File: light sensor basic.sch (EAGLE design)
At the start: 1 part

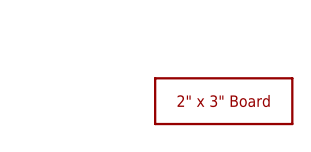
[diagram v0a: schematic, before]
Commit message: test
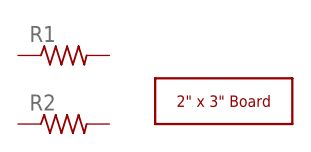
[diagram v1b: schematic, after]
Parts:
- added R1, R2: (no value), rcl:R-US_R1206
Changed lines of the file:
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@@
 <parts>
 <part name="U$1" library="voltera_community_lib" deviceset="2X3_BOARD" device="_V2"/>
+<part name="R1" library="rcl" library_urn="urn:adsk.eagle:library:334" deviceset="R-US_" device="R1206" package3d_urn="urn:adsk.eagle:package:23540/2"/>
+<part name="R2" library="rcl" library_urn="urn:adsk.eagle:library:334" deviceset="R-US_" device="R1206" package3d_urn="urn:adsk.eagle:package:23540/2"/>
 </parts>
 <sheets>
@@
 <instances>
 <instance part="U$1" gate="G$1" x="25.4" y="25.4" smashed="yes"/>
+<instance part="R1" gate="G$1" x="7.62" y="30.48" smashed="yes">
+<attribute name="NAME" x="3.81" y="31.9786" size="1.778" layer="95"/>
+<attribute name="VALUE" x="3.81" y="27.178" size="1.778" layer="96"/>
+</instance>
+<instance part="R2" gate="G$1" x="7.62" y="22.86" smashed="yes">
+<attribute name="NAME" x="3.81" y="24.3586" size="1.778" layer="95"/>
+<attribute name="VALUE" x="3.81" y="19.558" size="1.778" layer="96"/>
+</instance>
 </instances>
 <busses>
@@
 </schematic>
 </drawing>
+<compatibility>
+<note version="8.2" severity="warning">
+Since Version 8.2, EAGLE supports online libraries. The ids
+of those online libraries will not be understood (or retained)
+with this version.
+</note>
+<note version="8.3" severity="warning">
+Since Version 8.3, EAGLE supports URNs for individual library
+assets (packages, symbols, and devices). The URNs of those assets
+will not be understood (or retained) with this version.
+</note>
+<note version="8.3" severity="warning">
+Since Version 8.3, EAGLE supports the association of 3D packages
+with devices in libraries, schematics, and board files. Those 3D
+packages will not be understood (or retained) with this version.
+</note>
+<note version="8.4" severity="warning">
+Since Version 8.4, EAGLE supports properties for SPICE simulation.
+Probes in schematics and SPICE mapping objects found in parts and library devices
+will not be understood with this version. Update EAGLE to the latest version
+for full support of SPICE simulation.
+</note>
+</compatibility>
 </eagle>

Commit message: new test
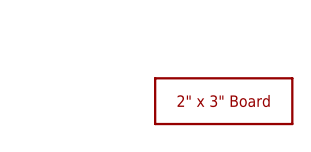
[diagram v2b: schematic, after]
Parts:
- removed R1, R2: (no value), rcl:R-US_R1206
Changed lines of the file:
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@@
 <parts>
 <part name="U$1" library="voltera_community_lib" deviceset="2X3_BOARD" device="_V2"/>
-<part name="R1" library="rcl" library_urn="urn:adsk.eagle:library:334" deviceset="R-US_" device="R1206" package3d_urn="urn:adsk.eagle:package:23540/2"/>
-<part name="R2" library="rcl" library_urn="urn:adsk.eagle:library:334" deviceset="R-US_" device="R1206" package3d_urn="urn:adsk.eagle:package:23540/2"/>
 </parts>
 <sheets>
@@
 <instances>
 <instance part="U$1" gate="G$1" x="25.4" y="25.4" smashed="yes"/>
-<instance part="R1" gate="G$1" x="7.62" y="30.48" smashed="yes">
-<attribute name="NAME" x="3.81" y="31.9786" size="1.778" layer="95"/>
-<attribute name="VALUE" x="3.81" y="27.178" size="1.778" layer="96"/>
-</instance>
-<instance part="R2" gate="G$1" x="7.62" y="22.86" smashed="yes">
-<attribute name="NAME" x="3.81" y="24.3586" size="1.778" layer="95"/>
-<attribute name="VALUE" x="3.81" y="19.558" size="1.778" layer="96"/>
-</instance>
 </instances>
 <busses>
@@
 </schematic>
 </drawing>
-<compatibility>
-<note version="8.2" severity="warning">
-Since Version 8.2, EAGLE supports online libraries. The ids
-of those online libraries will not be understood (or retained)
-with this version.
-</note>
-<note version="8.3" severity="warning">
-Since Version 8.3, EAGLE supports URNs for individual library
-assets (packages, symbols, and devices). The URNs of those assets
-will not be understood (or retained) with this version.
-</note>
-<note version="8.3" severity="warning">
-Since Version 8.3, EAGLE supports the association of 3D packages
-with devices in libraries, schematics, and board files. Those 3D
-packages will not be understood (or retained) with this version.
-</note>
-<note version="8.4" severity="warning">
-Since Version 8.4, EAGLE supports properties for SPICE simulation.
-Probes in schematics and SPICE mapping objects found in parts and library devices
-will not be understood with this version. Update EAGLE to the latest version
-for full support of SPICE simulation.
-</note>
-</compatibility>
 </eagle>
